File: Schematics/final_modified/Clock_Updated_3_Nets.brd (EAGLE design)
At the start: 50.8 x 50.8 mm, 51 parts, among them U1 ATMEGA328P, U2 V_REG_317DPACK

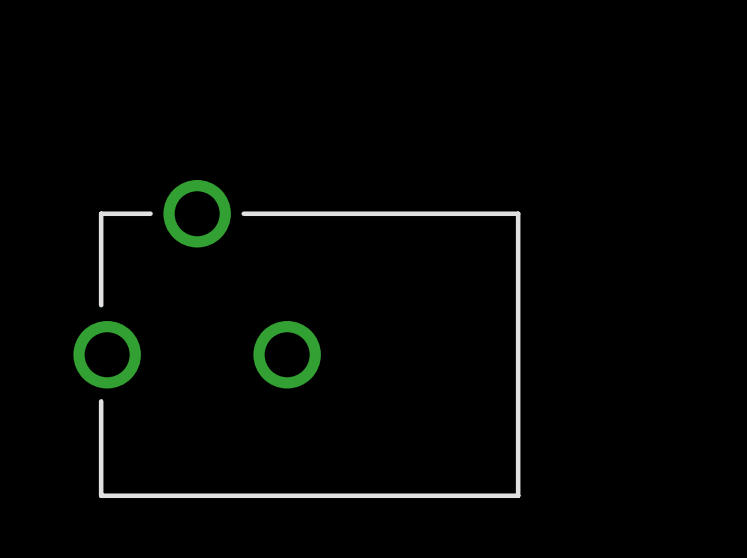
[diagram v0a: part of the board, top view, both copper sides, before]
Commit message: added test files
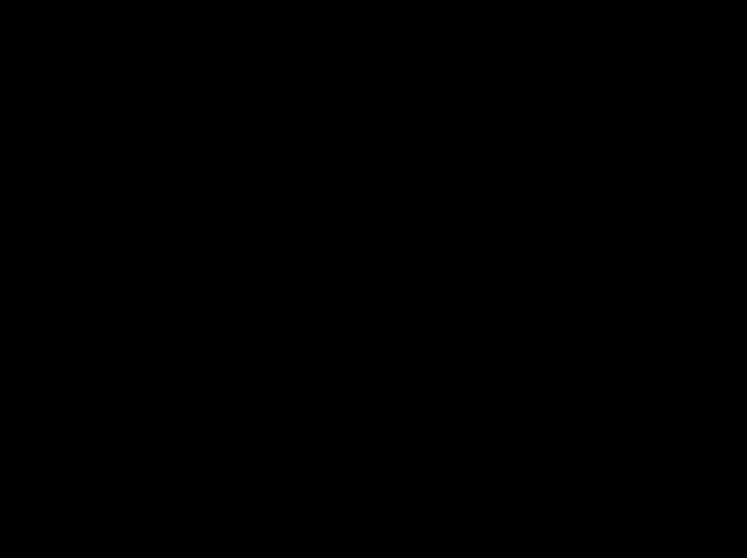
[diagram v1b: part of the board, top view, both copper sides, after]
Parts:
- removed U$2: CUI_PJ-102A, con-dc-jack:CUI_DCJACK_PCB
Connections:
- net N$45: no longer U$2.-
- net N$56: no longer U$2.+
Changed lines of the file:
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@@
 <?xml version="1.0" encoding="utf-8"?>
 <!DOCTYPE eagle SYSTEM "eagle.dtd">
-<eagle version="7.1.0">
+<eagle version="7.2.0">
 <drawing>
 <settings>
@@
 <attribute name="PROD_ID" value="RES-08788" x="-33.02" y="-105.664" size="1.778" layer="27" display="off"/>
 </element>
-<element name="U$2" library="con-dc-jack" package="CUI_DCJACK_PCB" value="CUI_PJ-102A" x="4.572" y="-128.016"/>
 </elements>
 <signals>
@@
 <wire x1="20.3454" y1="3.6576" x2="21.9456" y2="2.0574" width="0.254" layer="1"/>
 <wire x1="29.0322" y1="3.8862" x2="29.204" y2="4.09" width="0.254" layer="1"/>
-<contactref element="U$2" pad="-"/>
-<wire x1="21.9456" y1="2.0574" x2="7.572" y2="-128.016" width="0" layer="19" extent="1-1"/>
 </signal>
 <signal name="N$2">
@@
 <signal name="N$56">
 <contactref element="C15" pad="2"/>
-<contactref element="U$2" pad="+"/>
-<wire x1="20.32" y1="3.68" x2="1.572" y2="-128.016" width="0" layer="19" extent="1-1"/>
 </signal>
 </signals>
